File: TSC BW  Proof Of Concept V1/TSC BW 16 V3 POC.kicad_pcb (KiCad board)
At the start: 2 copper layers, 177.4 x 113.6 mm, 232 parts, among them J1 691312510002, J10 Micro_SD_Card_Det_Hirose_DM3AT, J13 Analog Inputs, J14 USB_C_Receptacle_USB2.0_16P, J17 691312510002, J18 RJ45_Hanrun_HR911105A_Horizon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, J19 691312510002, J2 CR1220_S8411_45R, J3 Free GPIO !pull-up, J4 Free GPIO pull-up, J5 Terminal Plug, J7 Terminal Plug, Q1 BC817, Q10 NCE60P10K, Q11 NCE60P10K, Q14 NCE60P10K, Q15 NCE60P10K, Q18 NCE60P10K, Q19 NCE60P10K, Q2 AO3401A, Q20 SS8050, Q21 SS8050, Q6 NCE60P10K, Q7 NCE60P10K, SW1 SW_Push, SW2 SW_Push, U1 XL1509-5.0, U10 PC357C, U11 PC357C, U14 PC357C, U15 PC357C, U18 PC357C, U19 PC357C, U2 AMS1117-3.3, U20 PCF8574T, U24 PC357C, U25 PC357C, U28 PC357C, U29 PC357C, U3 ESP32-S3-WROOM-1, U32 PC357C, U33 PC357C, U36 PC357C, U37 PC357C, U38 PCF8574T, U40 AT24CS04-SSHM, U41 DS3231MZ, U44 CH340C, U46 W5500, U48 MAX13487EESA, U6 PC357C, U7 PC357C, Y4 25M

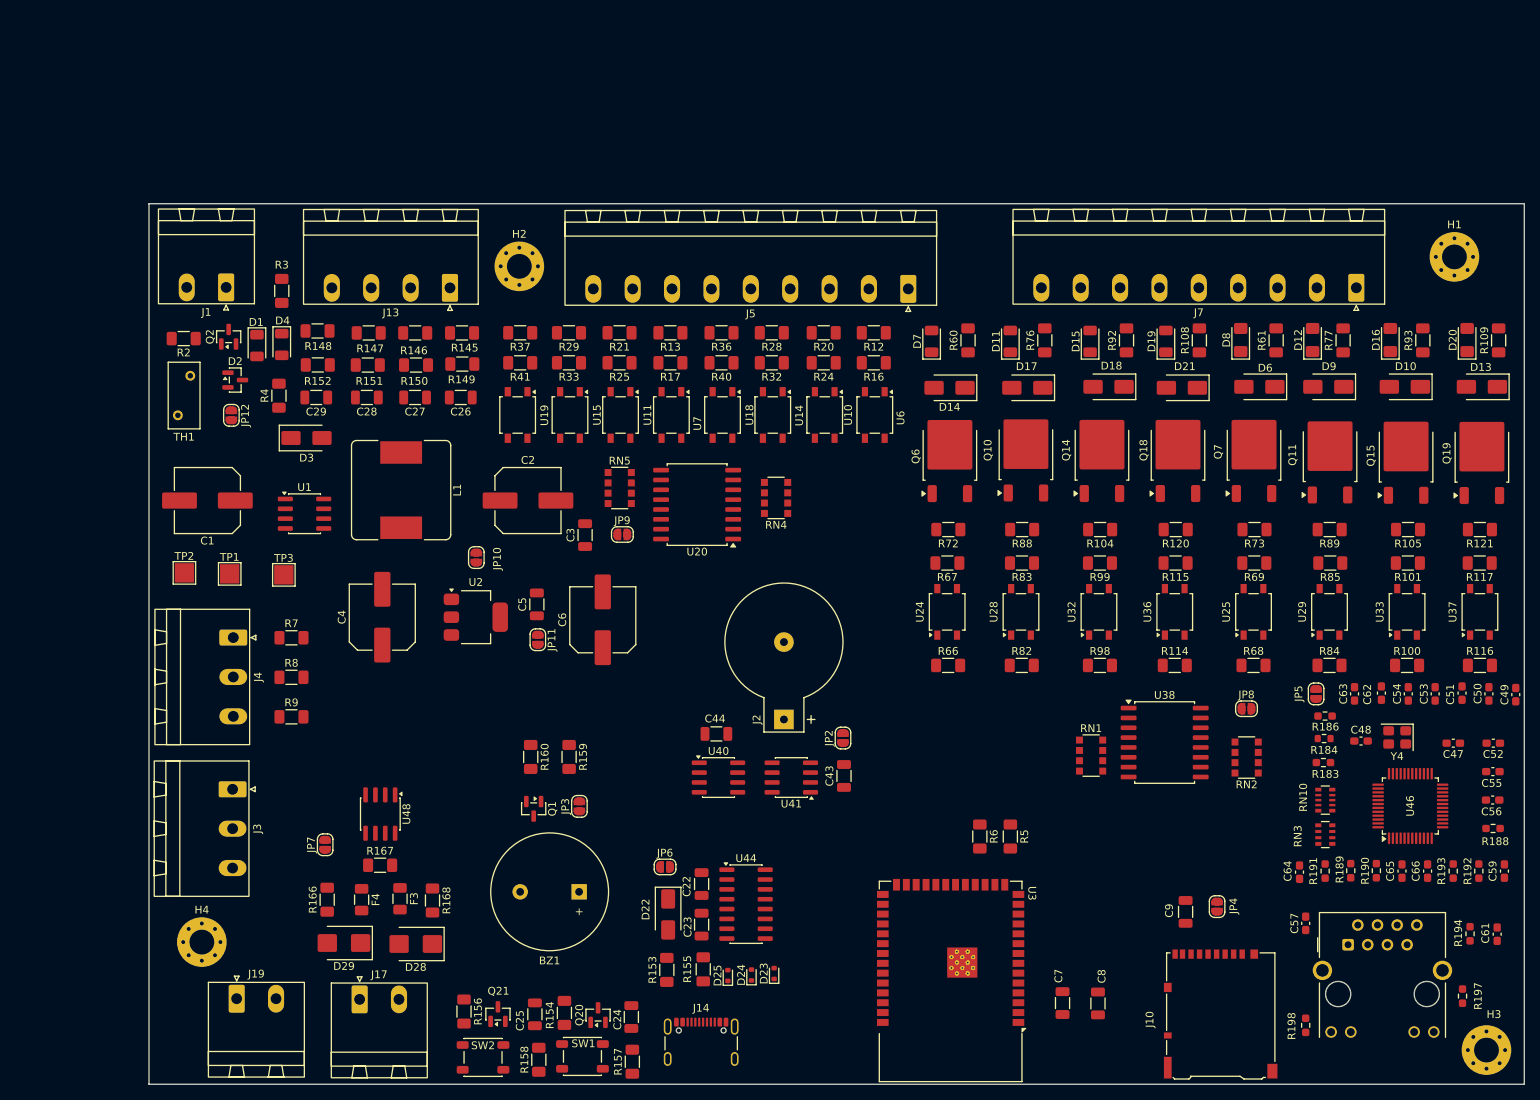
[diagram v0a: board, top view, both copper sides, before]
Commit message: WORKING ON POC - Proof of concept
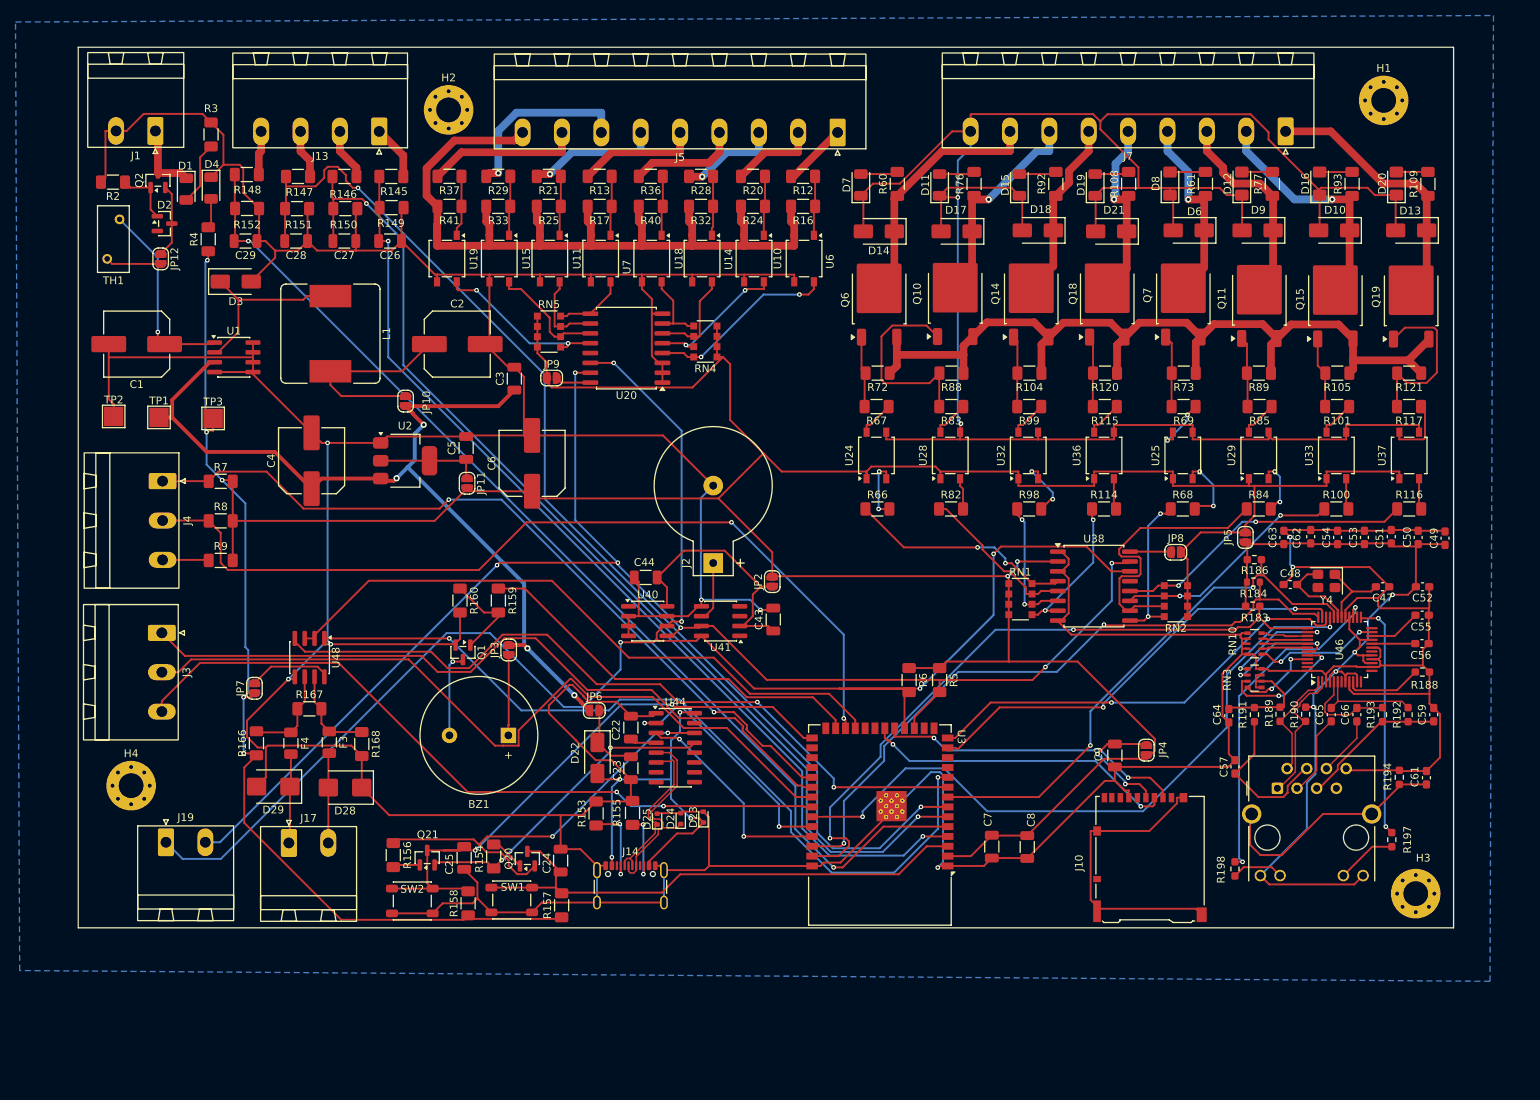
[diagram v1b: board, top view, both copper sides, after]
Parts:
- moved JP4 22.1 mm to (188.7, 111.9)
- moved R153 22.1 mm to (117.8, 120.1)
- moved D25 22.1 mm to (125.6, 120.8)
- moved C27 22.1 mm to (85.3, 46.2)
- moved C28 22.1 mm to (79.1, 46.2)
- moved C43 22.1 mm to (140.6, 95.0)
- moved C47 22.1 mm to (219.2, 90.8)
- moved C48 22.1 mm to (207.3, 90.5)
- moved C50 22.1 mm to (223.8, 84.5)
- moved C52 22.1 mm to (224.4, 90.8)
- moved C53 22.1 mm to (216.9, 84.5)
- moved C59 22.1 mm to (225.8, 107.3)
- moved C64 22.1 mm to (199.4, 107.5)
- moved C66 22.1 mm to (215.9, 107.3)
- moved D12 22.1 mm to (201.1, 38.8)
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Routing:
- net GND: track 0.00 -> 872.0 mm, vias 0 -> 8
- net +3V3: track 0.00 -> 519.2 mm, vias 0 -> 7
- net PGND: track 0.00 -> 281.7 mm, vias 0 -> 2
- net SCL: track 0.00 -> 222.4 mm, vias 0 -> 5
- net SDA: track 0.00 -> 188.5 mm, vias 0 -> 6
- net ANALOG_A3: track 0.00 -> 148.5 mm, vias 0 -> 2
- net ANALOG_A4: track 0.00 -> 139.6 mm, vias 0 -> 2
- net ANALOG_A2: track 0.00 -> 138.4 mm, vias 0 -> 2
- net +3V3 VW: track 0.00 -> 135.9 mm, vias 0 -> 4
- net ANALOG_A1: track 0.00 -> 128.7 mm, vias 0 -> 2
- net +5V: track 0.00 -> 115.3 mm, vias 0 -> 4
- net /ESP32 S3 MCU/F_IO47: track 0.00 -> 113.5 mm, vias 0 -> 2
- net VinLoad1: track 0.00 -> 113.2 mm
- net /8 DIGITAL INPUTS/PGND: track 0.00 -> 107.7 mm
- net 485RX: track 0.00 -> 104.7 mm, vias 0 -> 2
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- added copper zone on B.Cu, net GND
